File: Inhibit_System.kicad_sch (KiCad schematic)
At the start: 14 parts, among them Q10 Q_NMOS, Q11 Q_NMOS, Q12 Q_NMOS, Q13 Q_NMOS, Q2 Q_NMOS, Q7 Q_NMOS, Q9 Q_NMOS, SW2 SW_SPST, SW3 SW_SPST, SW4 SW_SPST

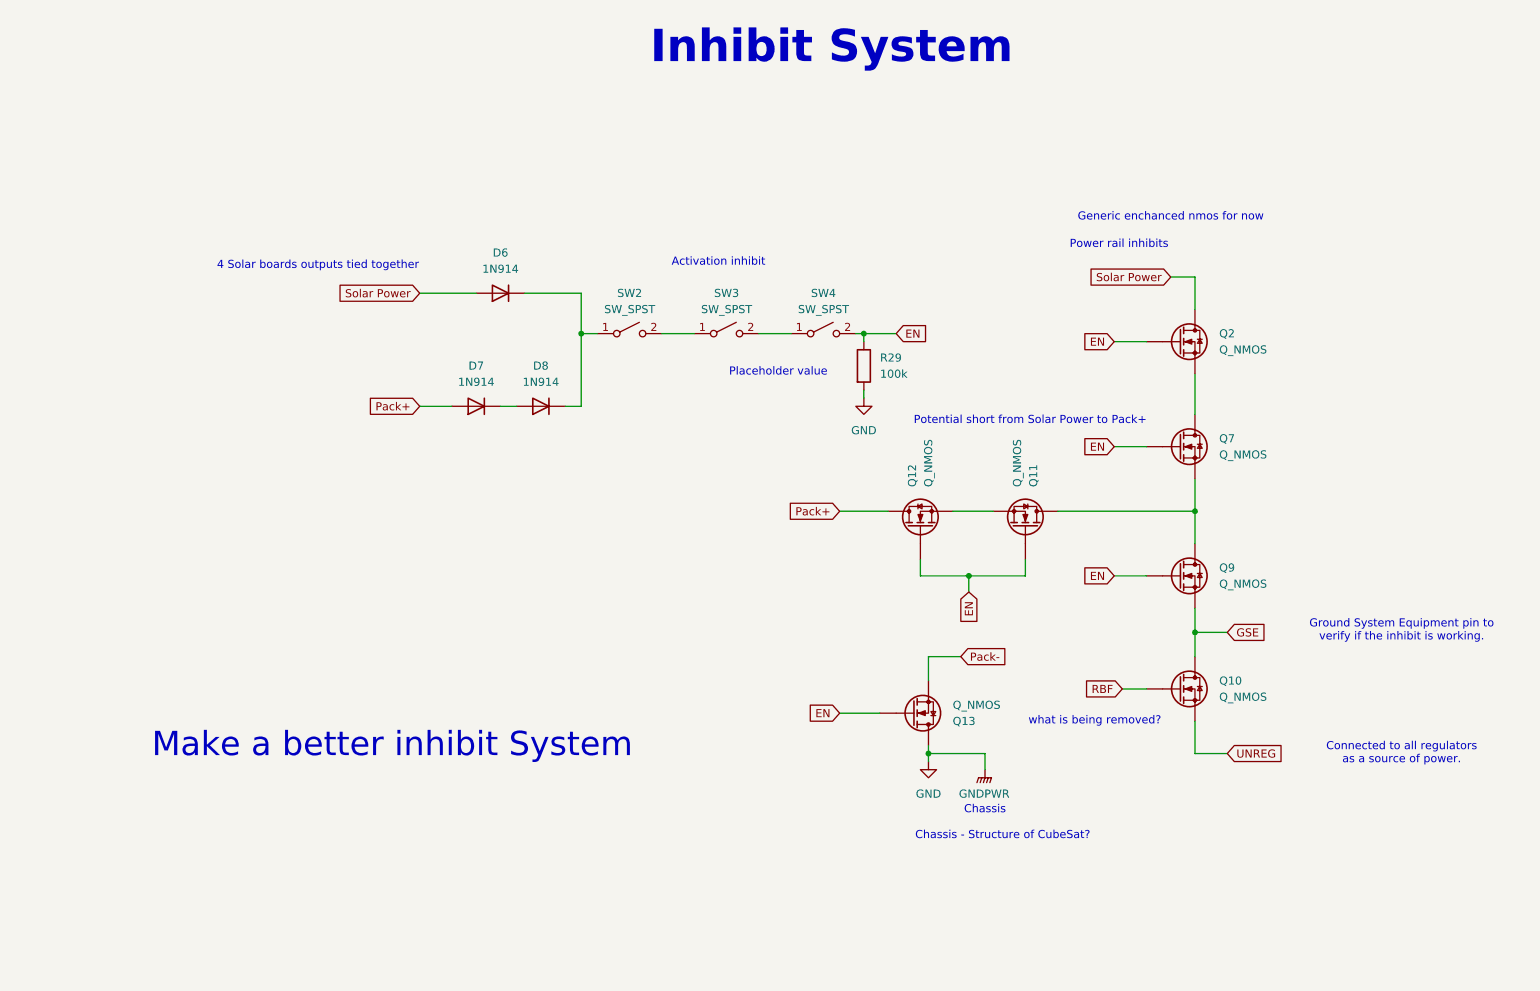
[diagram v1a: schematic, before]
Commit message: Updates to inhibit
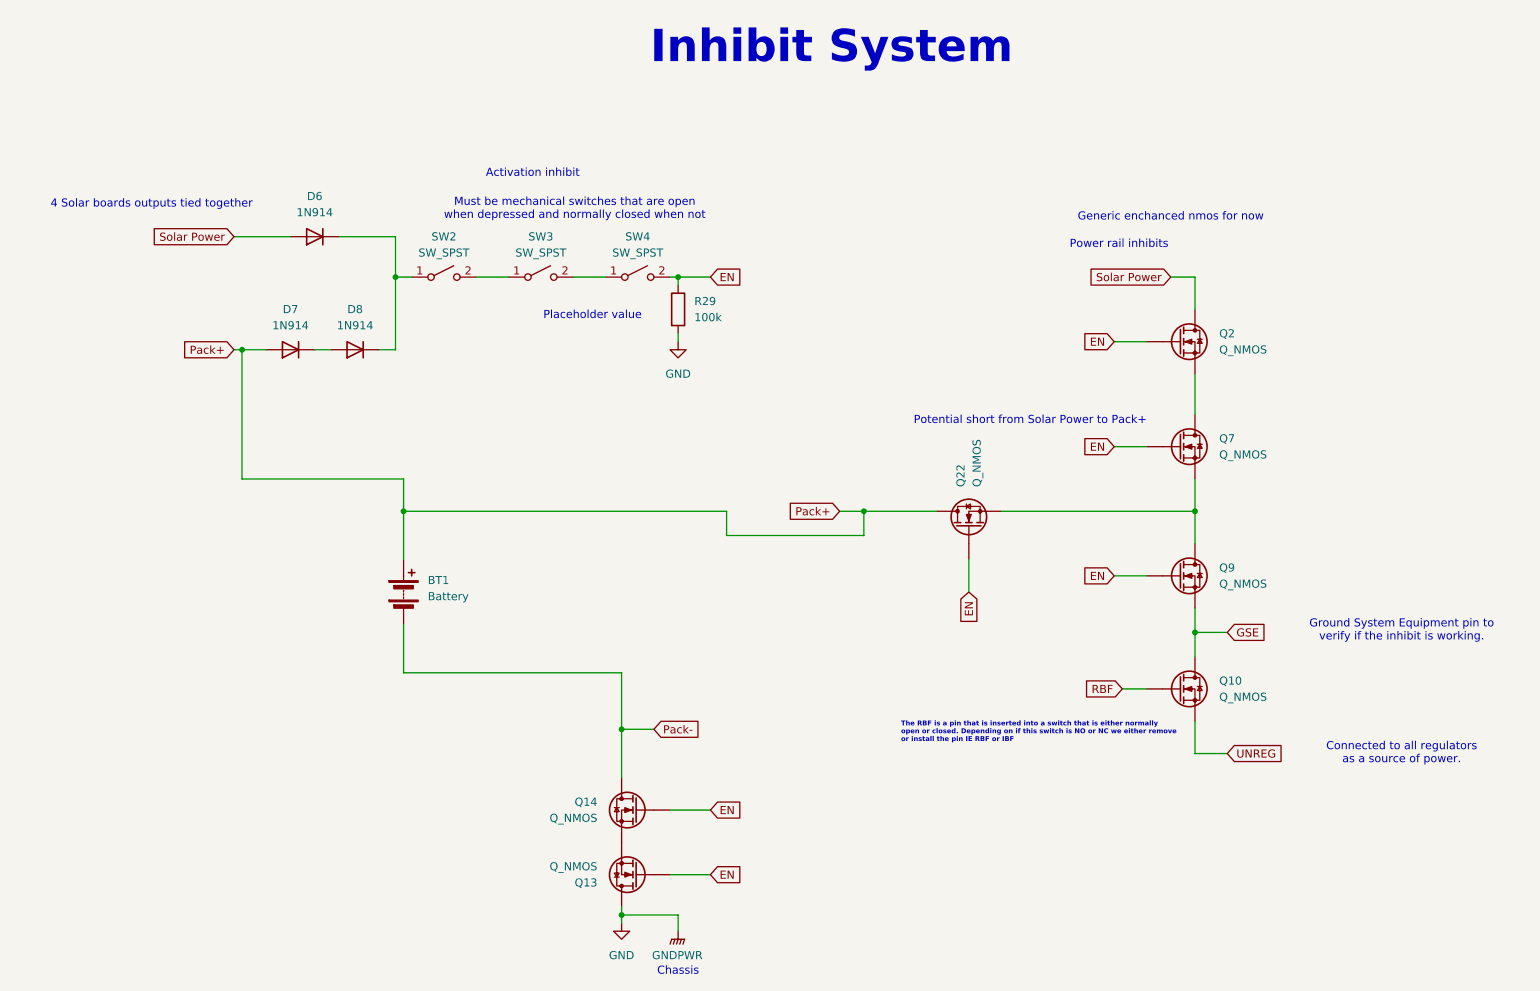
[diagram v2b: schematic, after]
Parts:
- removed Q11, Q12: Q_NMOS, symbol Device:Q_NMOS
- added BT1: Battery, symbol Device:Battery
- added Q14, Q22: Q_NMOS, symbol Device:Q_NMOS
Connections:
- net EN: now also Q14.G, Q22.G
- net Pack+: now also BT1.1 (+), Q22.D
- net Pack-: now also BT1.2 (-), Q14.D; no longer Q13.S
- net at Q7.S, Q9.D: now also Q22.S
- new net: Q13.S, Q14.S
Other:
- note added: "Must be mechanical switches that are open when depressed and normally closed when not"
- note added: "The RBF is a pin that is inserted into a switch that is either normally open or closed. Depending on if this switch is NO or NC we either remove or install the pin IE RBF or IBF"
- note removed: "Chassis - Structure of CubeSat?"
- note removed: "Make a better inhibit System"
- note removed: "what is being removed?"
- moved on the sheet: D6, D7, D8, Q13, R29, SW2, SW3, SW4
